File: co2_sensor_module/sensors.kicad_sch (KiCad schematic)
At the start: 11 parts, among them U1 SGX-7OX, U3 ADS1115IDGS, U5 MS5611-01BA, U6 SHT4x, U7 STC31-C

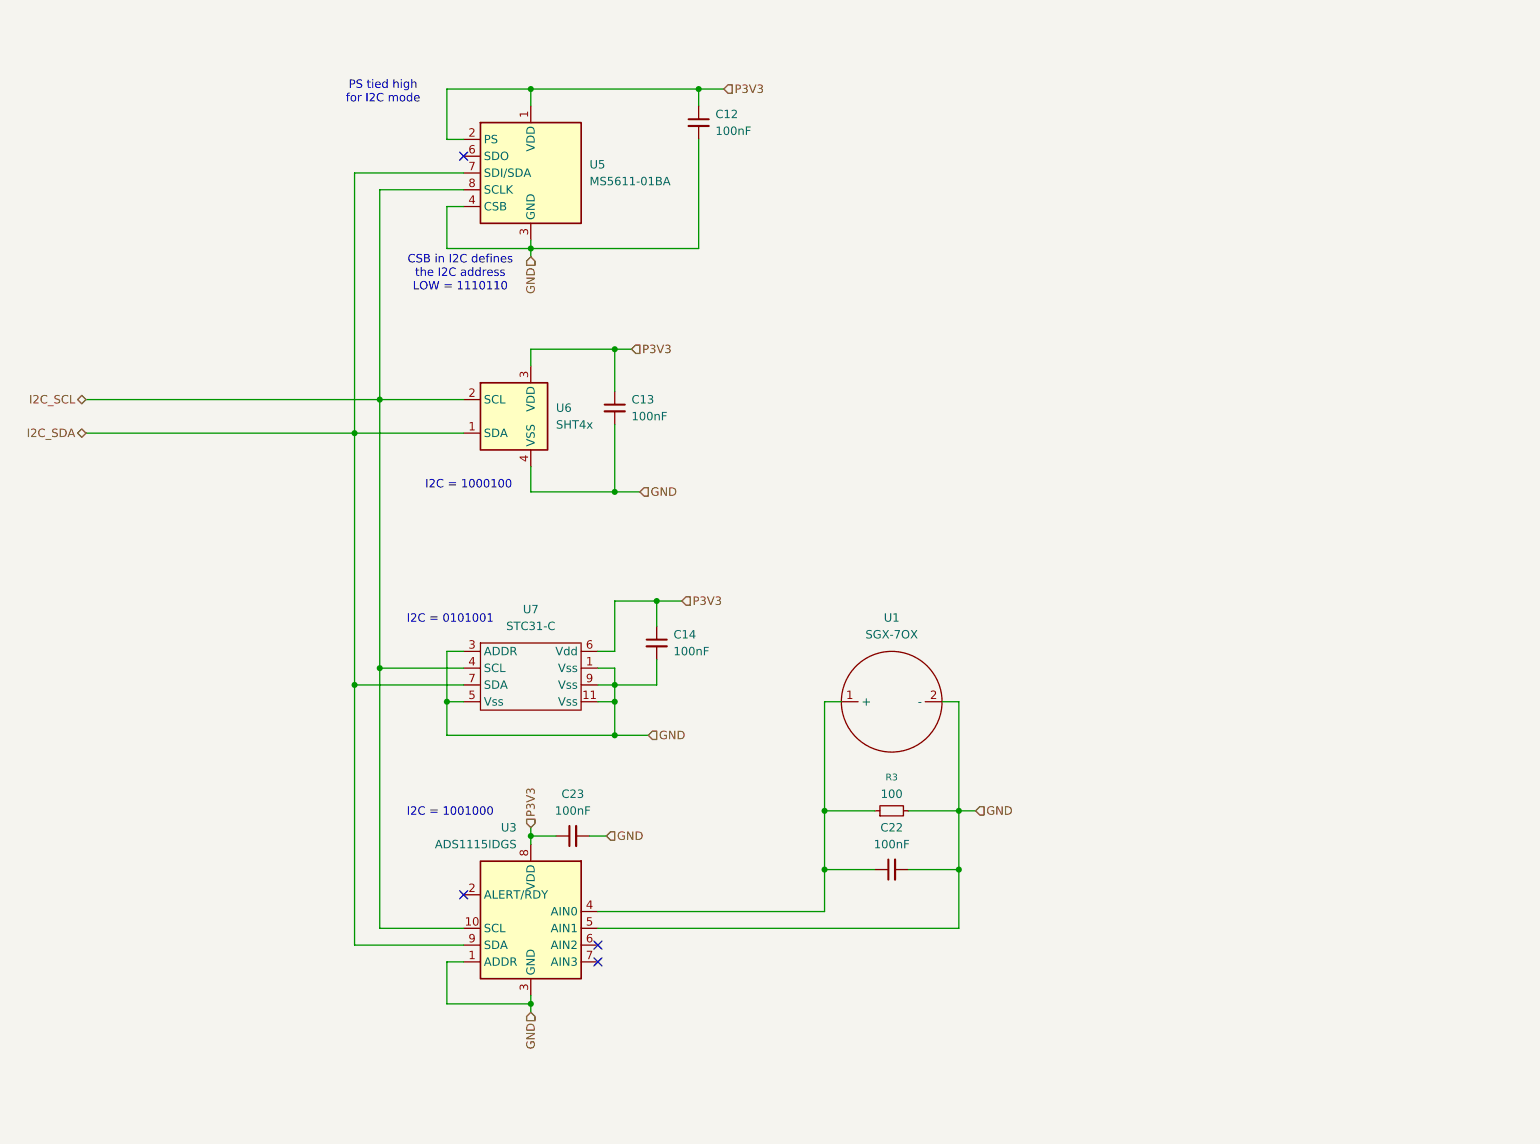
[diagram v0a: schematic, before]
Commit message: (mostly) finalized sensing units + progress on surface hub
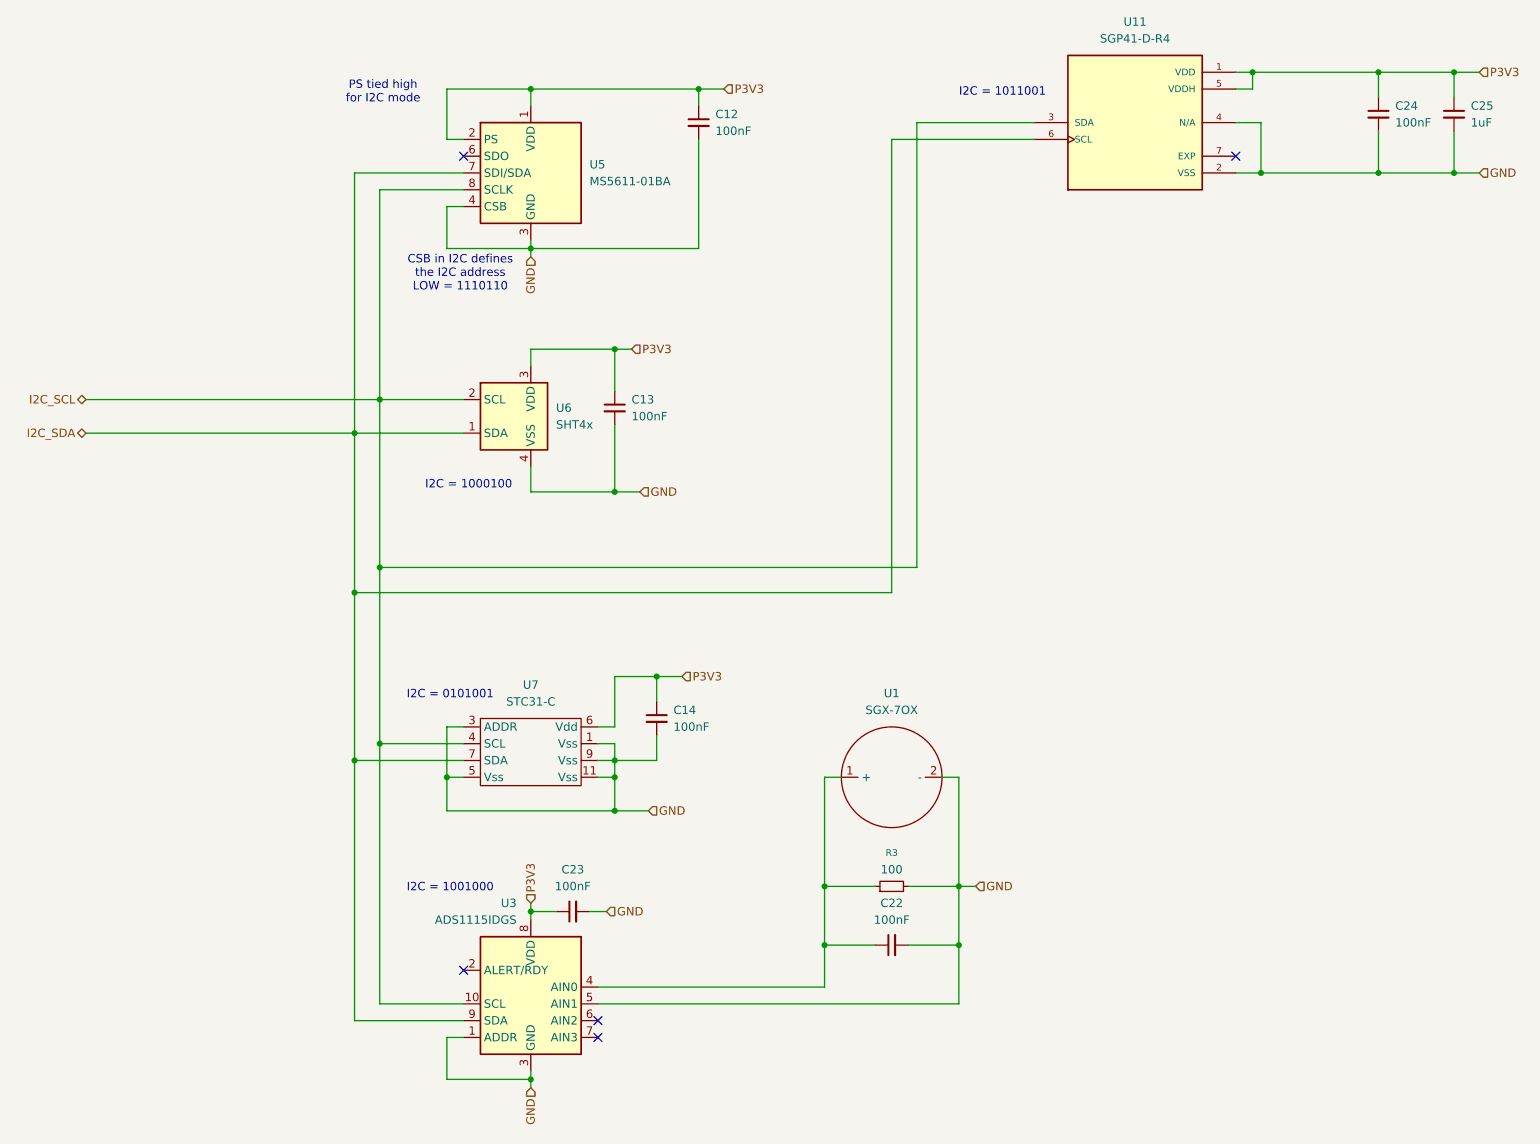
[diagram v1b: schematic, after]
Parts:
- added C24: 100nF, Capacitor_SMD:C_0402_1005Metric, symbol Device:C_Small
- added C25: 1uF, Capacitor_SMD:C_0603_1608Metric, symbol Device:C_Small
- added U11: SGP41-D-R4, CustomFootprints:XDCR_SGP41-D-R4, symbol CustomSymbols:SGP41-D-R4
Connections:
- net GND: now also C24.2, C25.2, U11.2 (VSS), U11.4 (N/A)
- net I2C_SCL: now also U11.3 (SDA)
- net I2C_SDA: now also U11.6 (SCL)
- net P3V3: now also C24.1, C25.1, U11.1 (VDD), U11.5 (VDDH)
- no-connect marks 4 -> 5
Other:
- note added: "I2C = 1011001"
- moved on the sheet: C14, C22, C23, R3, U1, U3, U7
